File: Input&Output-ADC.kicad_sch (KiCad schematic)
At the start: 47 parts, among them U2 G=1

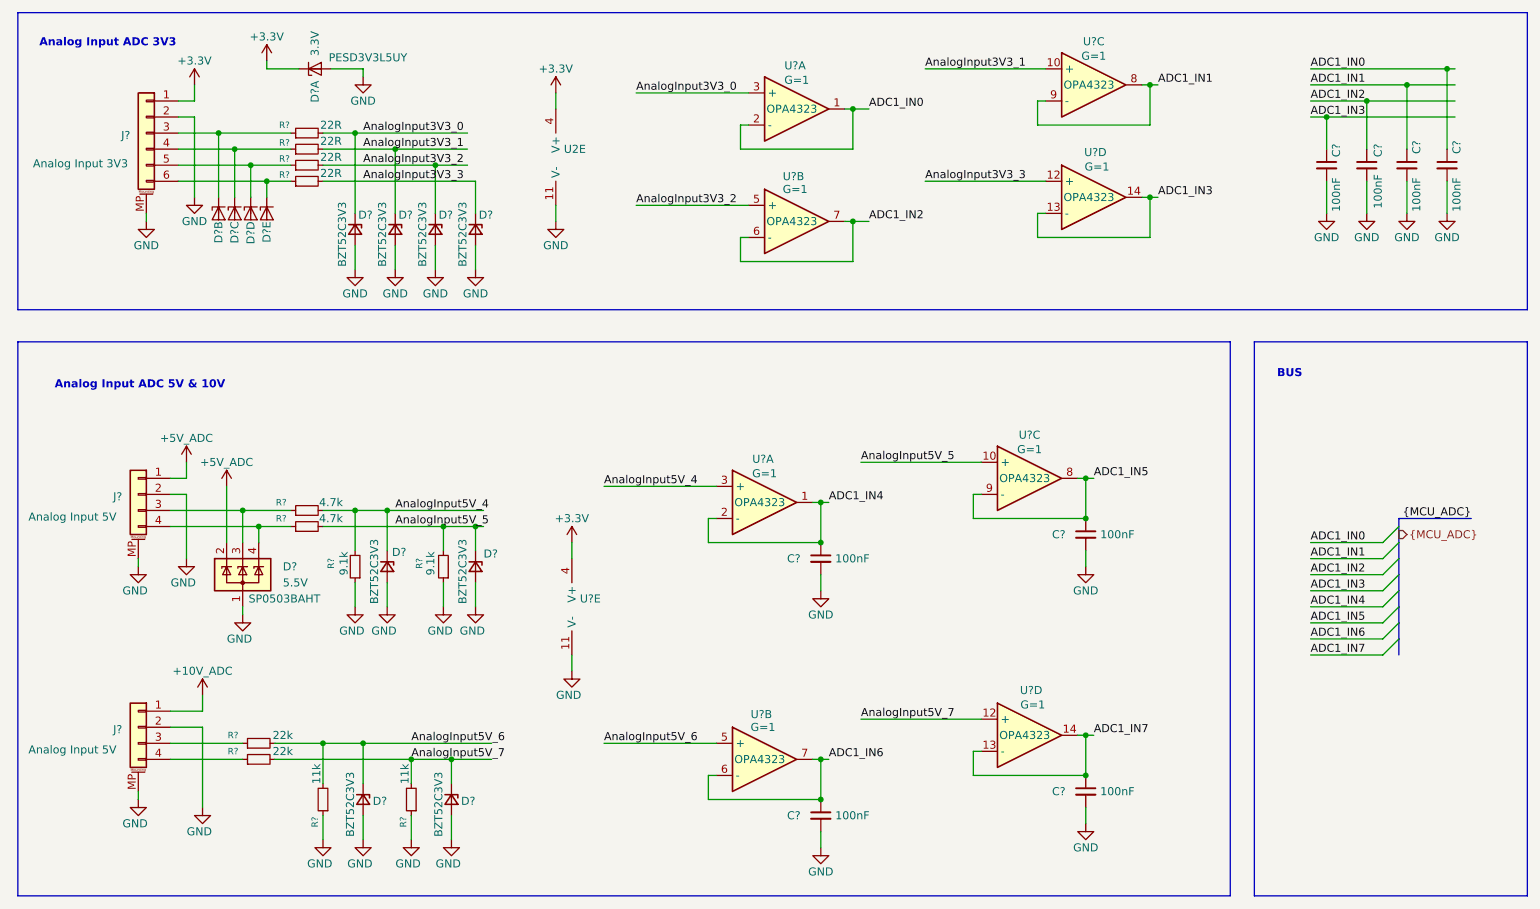
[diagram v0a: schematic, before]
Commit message: IOT part Finilization
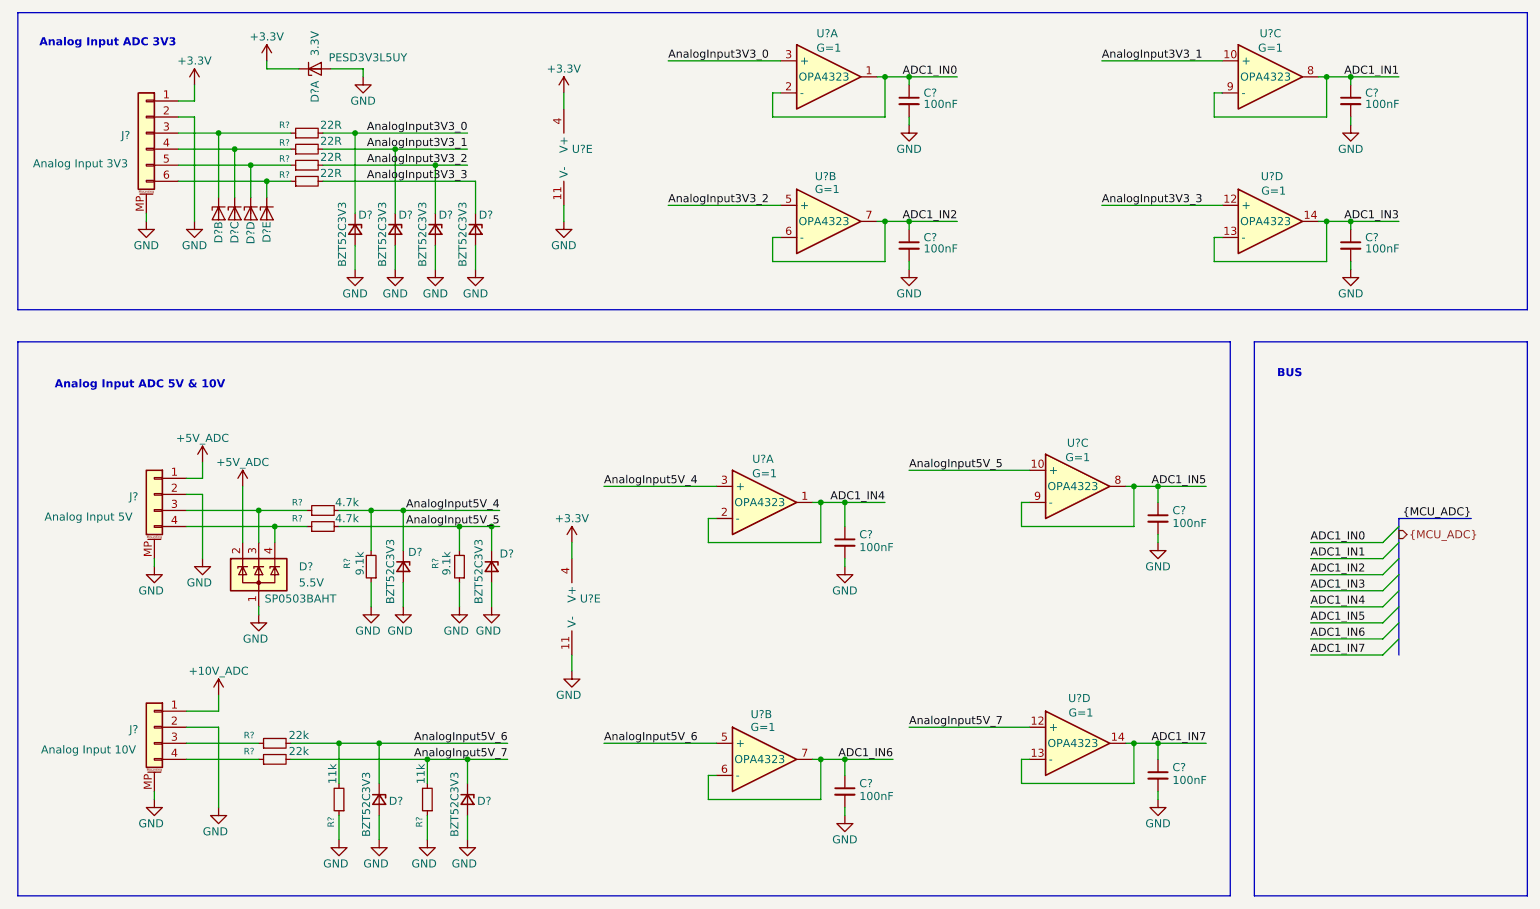
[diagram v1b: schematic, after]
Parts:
- removed C? (x8): 100nF, Capacitor_SMD:C_0603_1608Metric_Pad1.08x0.95mm_HandSolder, symbol Device:C_Small
- added C? (x8): 100nF, Capacitor_SMD:C_0603_1608Metric_Pad1.08x0.95mm_HandSolder, symbol Device:C_Small
- J?: Comment Analog Input 5V -> Analog Input 10V
- renumbered U2 to U?
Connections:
- net ADC1_IN0: now also C?.1
- net ADC1_IN1: now also C?.1
- net ADC1_IN2: now also C?.1
- net ADC1_IN3: now also C?.1
- net ADC1_IN4: now also C?.1
- net ADC1_IN5: now also C?.1
- net ADC1_IN6: now also C?.1
- net ADC1_IN7: now also C?.1
- net GND: now also C?.2, C?.2, C?.2, C?.2, C?.2, C?.2, C?.2, C?.2
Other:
- moved on the sheet: D?, J?, R?, U?A, U?B, U?C, U?D, U?E
